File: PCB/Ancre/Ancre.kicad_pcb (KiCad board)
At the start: 2 copper layers, 72.8 x 63 mm, 11 parts, among them IC1 TCAN1051VDRQ1, U1 OKI-78SR-5_1.5-W36-C, U2 DB301V-5.0-2P, U3 DB301V-5.0-2P

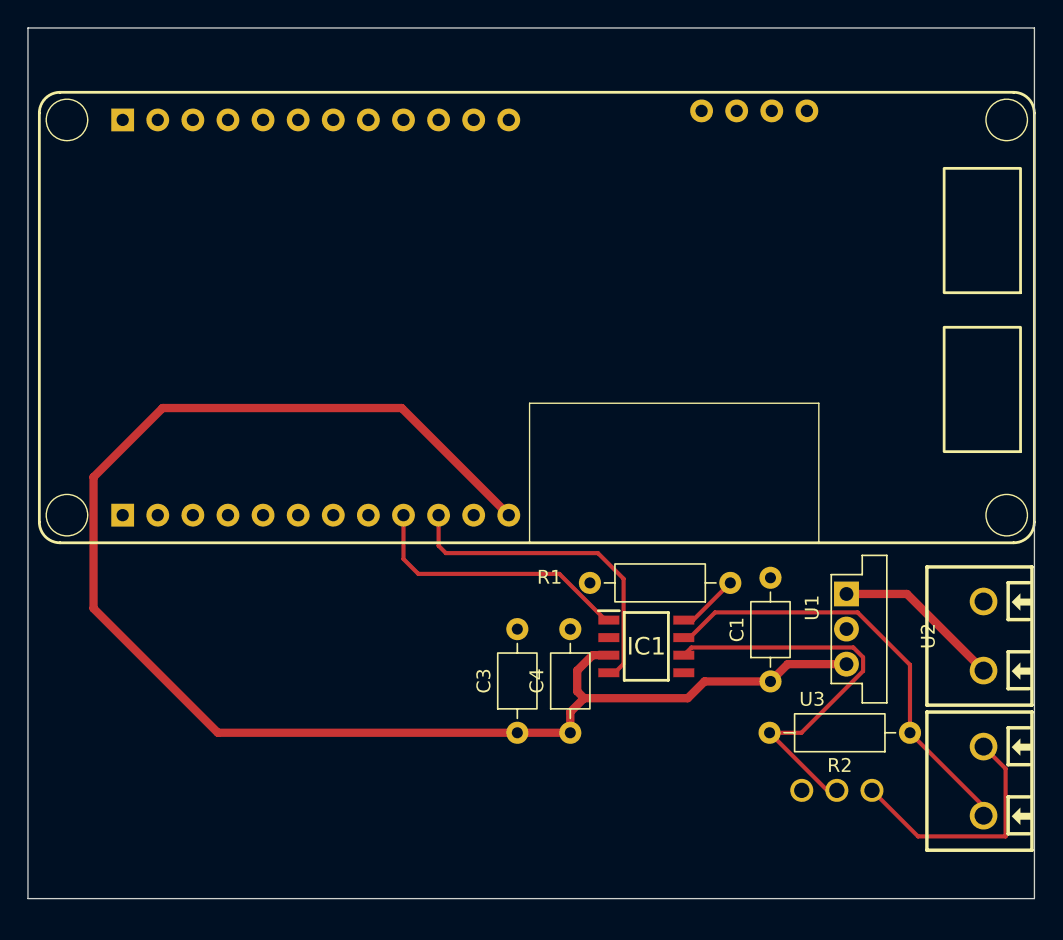
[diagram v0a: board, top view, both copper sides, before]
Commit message: MaJ PCB ancre pistes
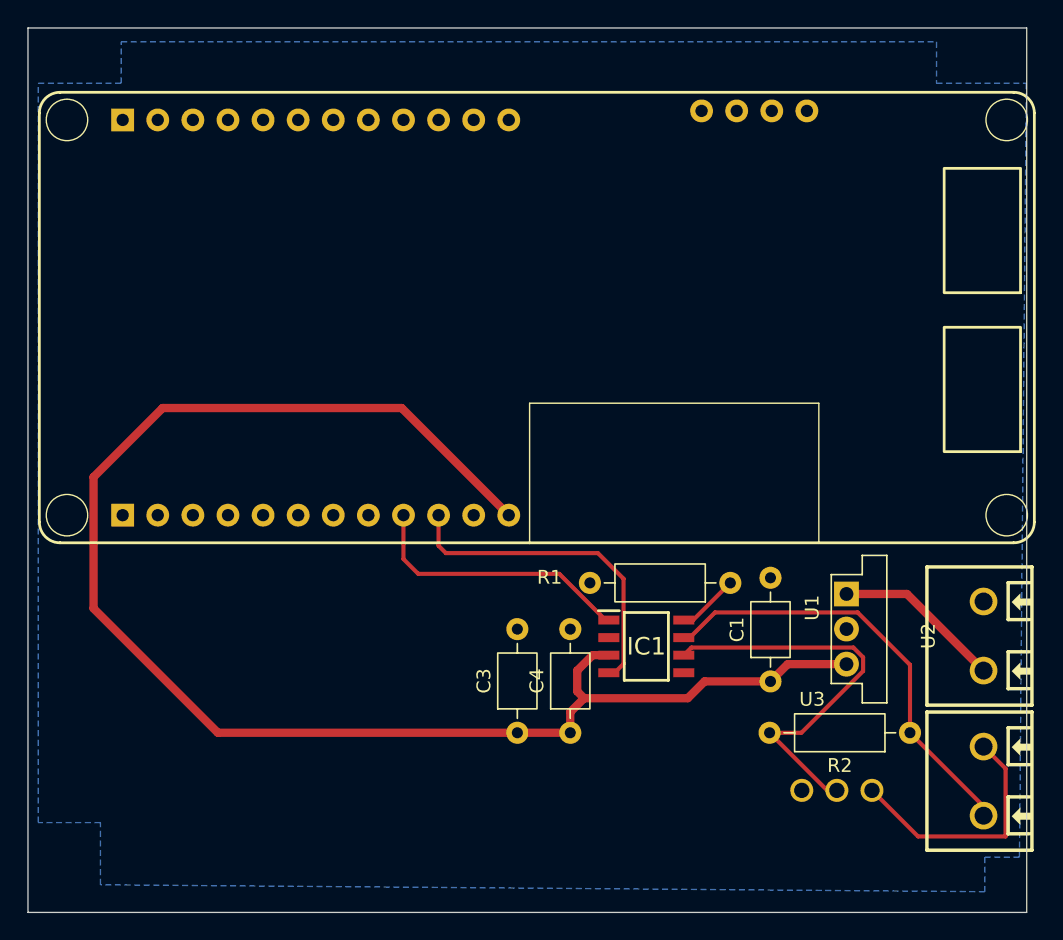
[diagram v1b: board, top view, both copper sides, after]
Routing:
- added copper zone on B.Cu, net GNDREF
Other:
- board size 72.8 x 63 mm -> 72.3 x 64 mm
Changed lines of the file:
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@@
 	(gr_rect
 		(start 149.756774 37.5)
-		(end 222.58595 100.5)
+		(end 222.02597 101.5)
 		(stroke
 			(width 0.05)
@@
 		(net "Net-(IC1-RXD)")
 	)
+	(zone
+		(net "GNDREF")
+		(layer "B.Cu")
+		(hatch edge 0.5)
+		(connect_pads
+			(clearance 0.5)
+		)
+		(min_thickness 0.25)
+		(fill yes
+			(thermal_gap 0.5)
+			(thermal_bridge_width 0.5)
+			(island_removal_mode 0)
+		)
+		(polygon
+			(pts
+				(xy 219 100) (xy 155 99.5) (xy 155 95) (xy 150.5 95) (xy 150.5 41.5) (xy 156.5 41.5) (xy 156.5 38.5)
+				(xy 215.5 38.5) (xy 215.5 41.5) (xy 222 41.5) (xy 221.5 97.5) (xy 219 97.5)
+			)
+		)
+	)
 	(embedded_fonts no)
